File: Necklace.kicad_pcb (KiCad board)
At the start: 2 copper layers, 29 parts, among them P1 PICOBLADE_5_HDR_RA, P2 PICOBLADE_5_HDR_RA, SW1 CK_KMR2, U1 ADXL345, U2 MSP430G2452IPW14

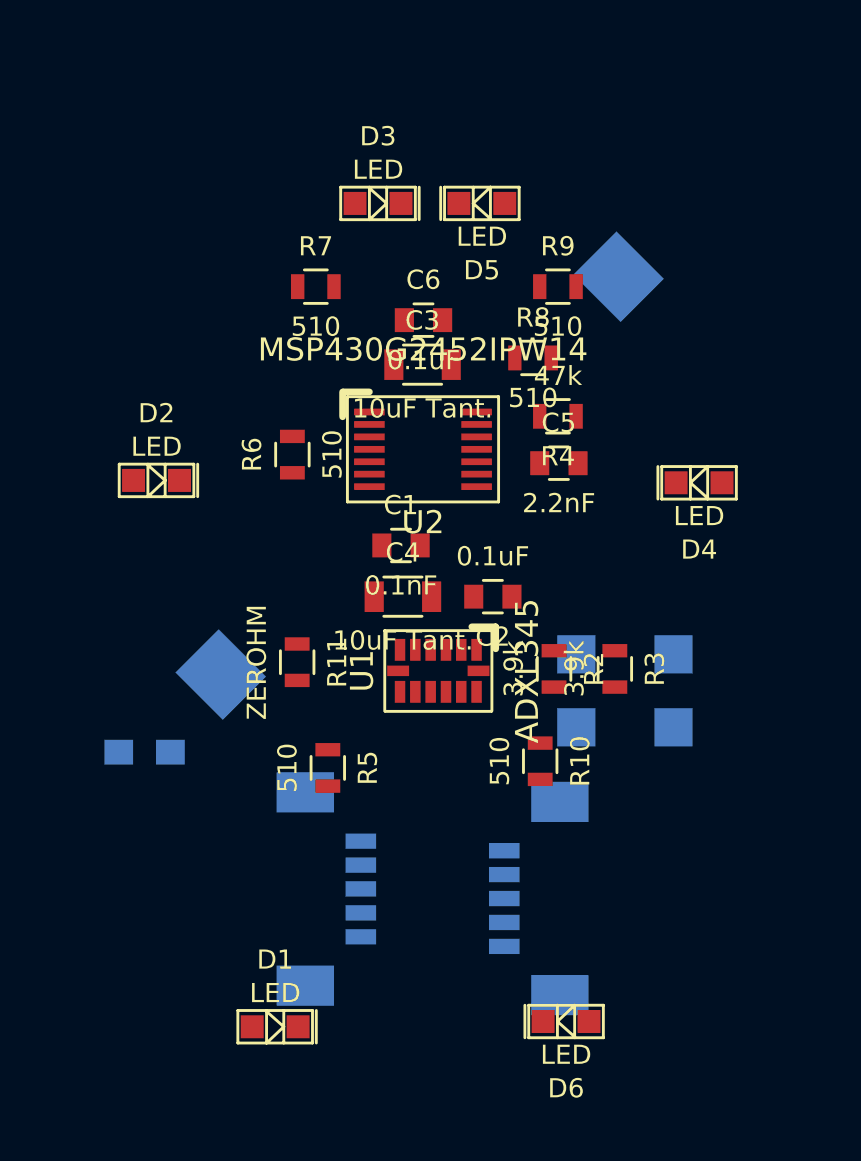
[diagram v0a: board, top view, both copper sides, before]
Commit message: and some more layout
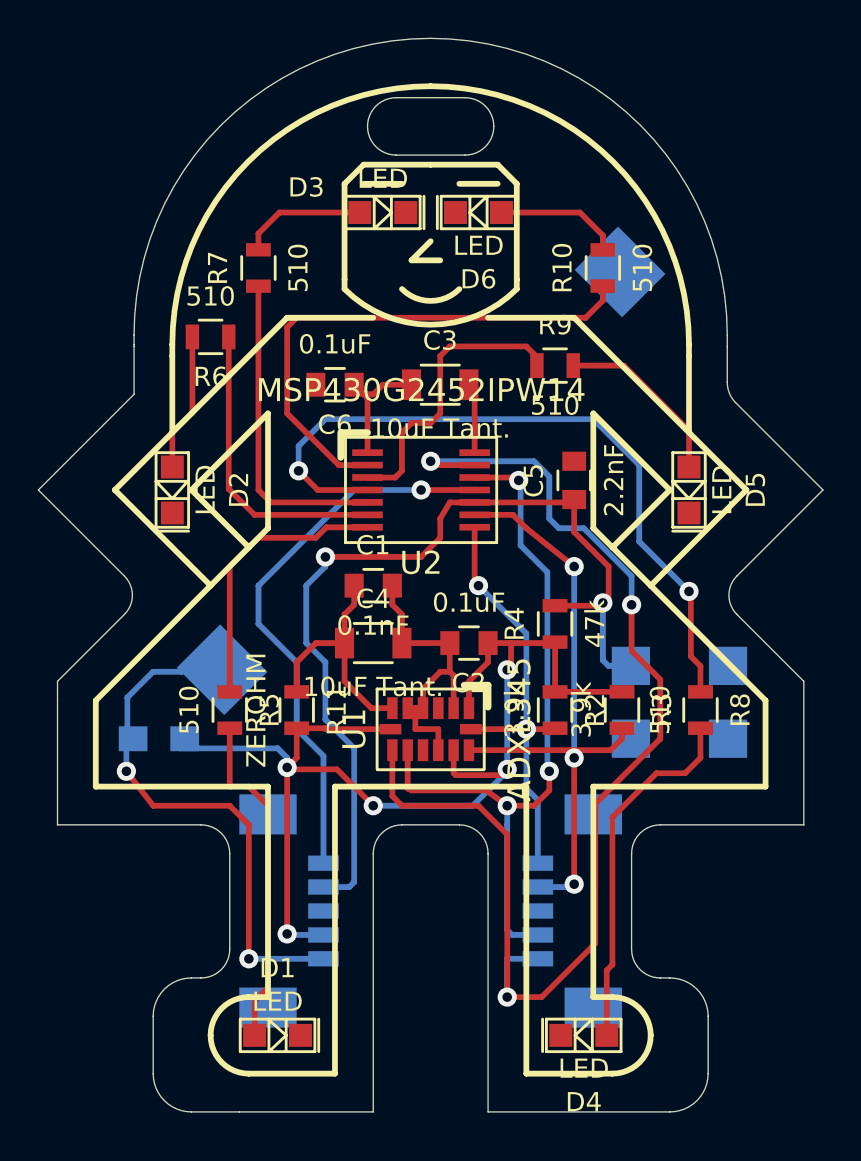
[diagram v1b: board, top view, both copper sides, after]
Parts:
- moved D6 42.5 mm to (115.0, 90.0)
- moved D4 29.5 mm to (120.5, 133.0)
- moved R10 26.0 mm to (121.5, 92.9), turned to 90 degrees
- moved R8 20.4 mm to (126.6, 116.0), turned to 270 degrees
- moved D5 18.5 mm to (126.0, 104.5), turned to 270 degrees
- moved R4 10.9 mm to (119.0, 111.5), turned to 90 degrees
- moved R6 7.49 mm to (101.0, 96.5), turned to 180 degrees
- moved R5 5.95 mm to (102.0, 116.0)
- moved C6 5.73 mm to (107.5, 99.0), turned to 180 degrees
- moved R9 4.13 mm to (119.0, 98.0)
- moved R7 3.15 mm to (103.5, 92.9), turned to 90 degrees
- moved U1 3.08 mm to (112.5, 117.0)
- moved SW1 2.91 mm to (125.5, 117.5)
- moved C4 2.88 mm to (109.5, 112.5)
- moved C2 2.73 mm to (114.5, 112.5)
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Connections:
- P2 pad 4: /ACC_INT1 -> /ACC_INT2
- P2 pad 5: /ACC_INT2 -> /ACC_INT1
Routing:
- net +BATT: track 0.00 -> 69.1 mm, vias 0 -> 5
- net /ACC_INT1: track 0.00 -> 65.0 mm, vias 0 -> 3
- net /SBWTDIO: track 0.00 -> 48.8 mm, vias 0 -> 2
- net Net-(R8-Pad1): track 0.00 -> 37.9 mm, vias 0 -> 2
- net /ACC_INT2: track 0.00 -> 37.4 mm, vias 0 -> 3
- net /I2C_SDA: track 0.00 -> 34.3 mm, vias 0 -> 3
- net /SBWTCK: track 0.00 -> 29.3 mm, vias 0 -> 1
- net Net-(BATT1-Pad2): track 0.00 -> 28.9 mm, vias 0 -> 2
- net Net-(R10-Pad1): track 0.00 -> 27.6 mm
- net /I2C_SCL: track 0.00 -> 23.3 mm, vias 0 -> 2
- net GND: track 0.00 -> 20.0 mm
- net Net-(D4-Pad1): track 0.00 -> 19.0 mm
- net Net-(D1-Pad1): track 0.00 -> 17.8 mm
- net Net-(R7-Pad1): track 0.00 -> 16.5 mm
- net Net-(R6-Pad1): track 0.00 -> 15.8 mm
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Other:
- board outline added: 41 x 56.1 mm
- net class Default: clearance 0.254 -> 0.3; trace_width 0.254 -> 0.3; via_dia 0.889 -> 1; via_drill 0.635 -> 0.6
- rule trace_clearance: 0.254 -> 0.3
